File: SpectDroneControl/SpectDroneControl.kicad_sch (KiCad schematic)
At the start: 125 parts, among them J1 Conn_02x03_Counter_Clockwise, J1-1 Conn_01x04_Male, J1-2 Conn_01x04_Male, J3-1 Conn_01x01_Female, J3-2 Conn_01x01_Female, J3-3 Conn_01x01_Female, J3-4 Conn_01x01_Female, J3-5 Conn_01x01_Female, J3V1 Conn_01x01_Male, J5-1 Conn_01x01_Female, J5-2 Conn_01x01_Female, J5-3 Conn_01x01_Female, J5-4 Conn_01x01_Female, J5-5 Conn_01x01_Female, Q1 FDN340P, SW1 SW_SPDT, U1 Teensy4.1, U2 Teensy4.0, U3 NVT2010PW, U4 NVT2010PW, U5 NVT2010PW, U6 MCP112-450E/TO, U7 LM7805_SOT223

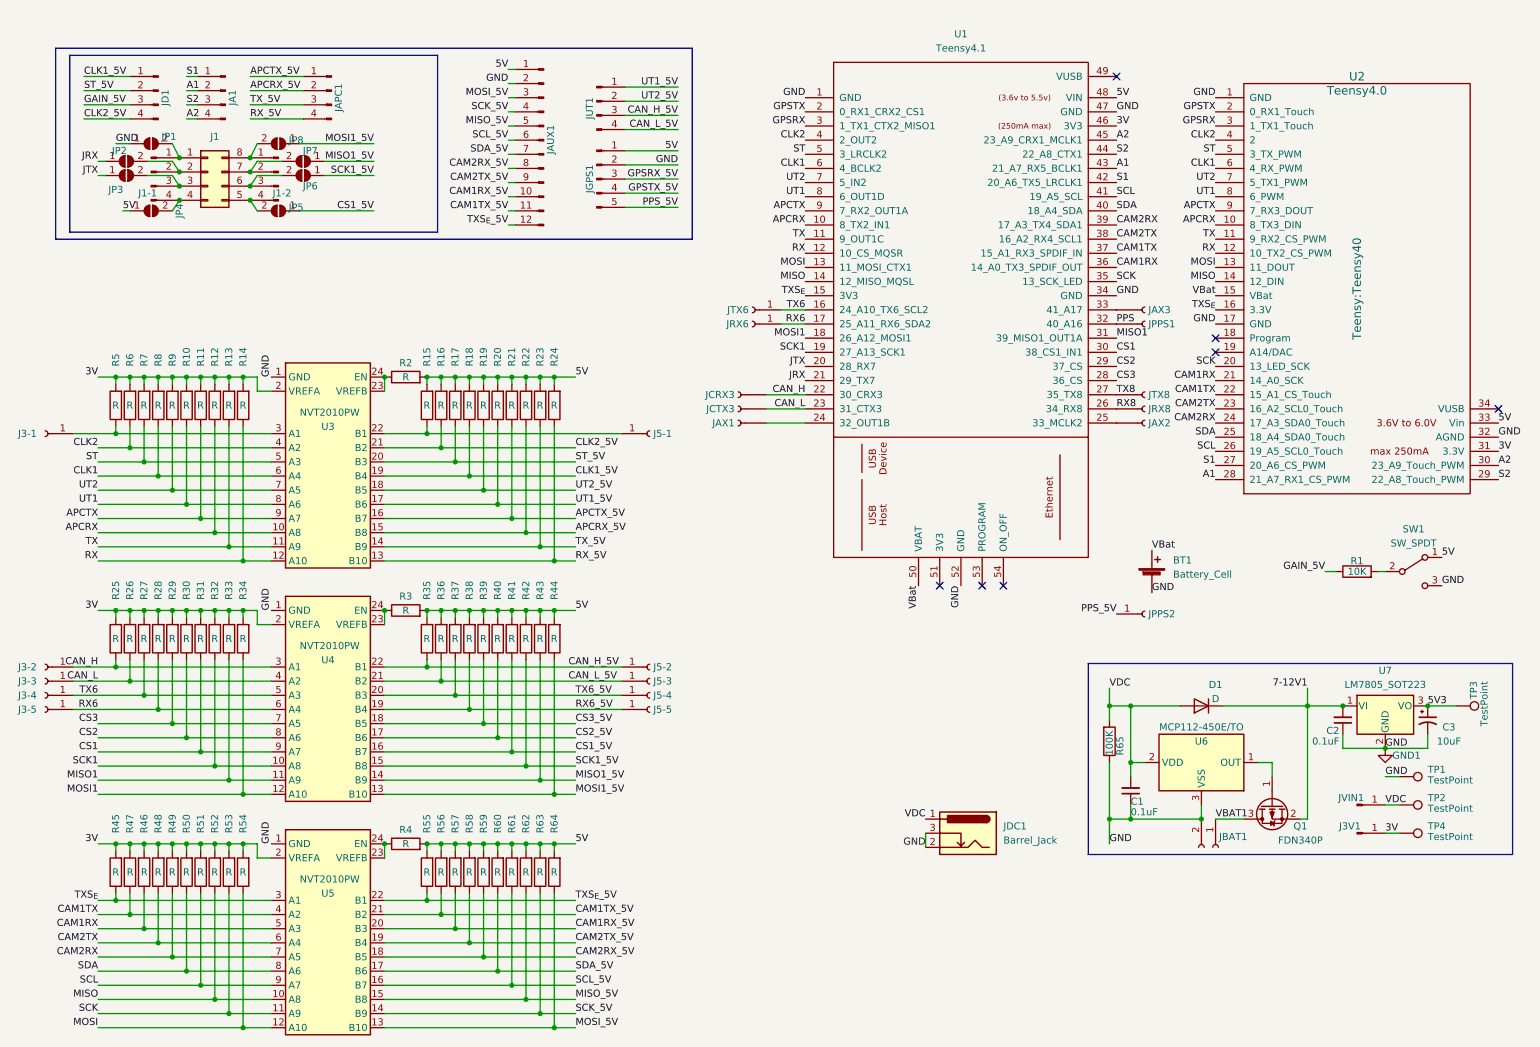
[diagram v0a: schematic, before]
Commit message: SpectDrone Development
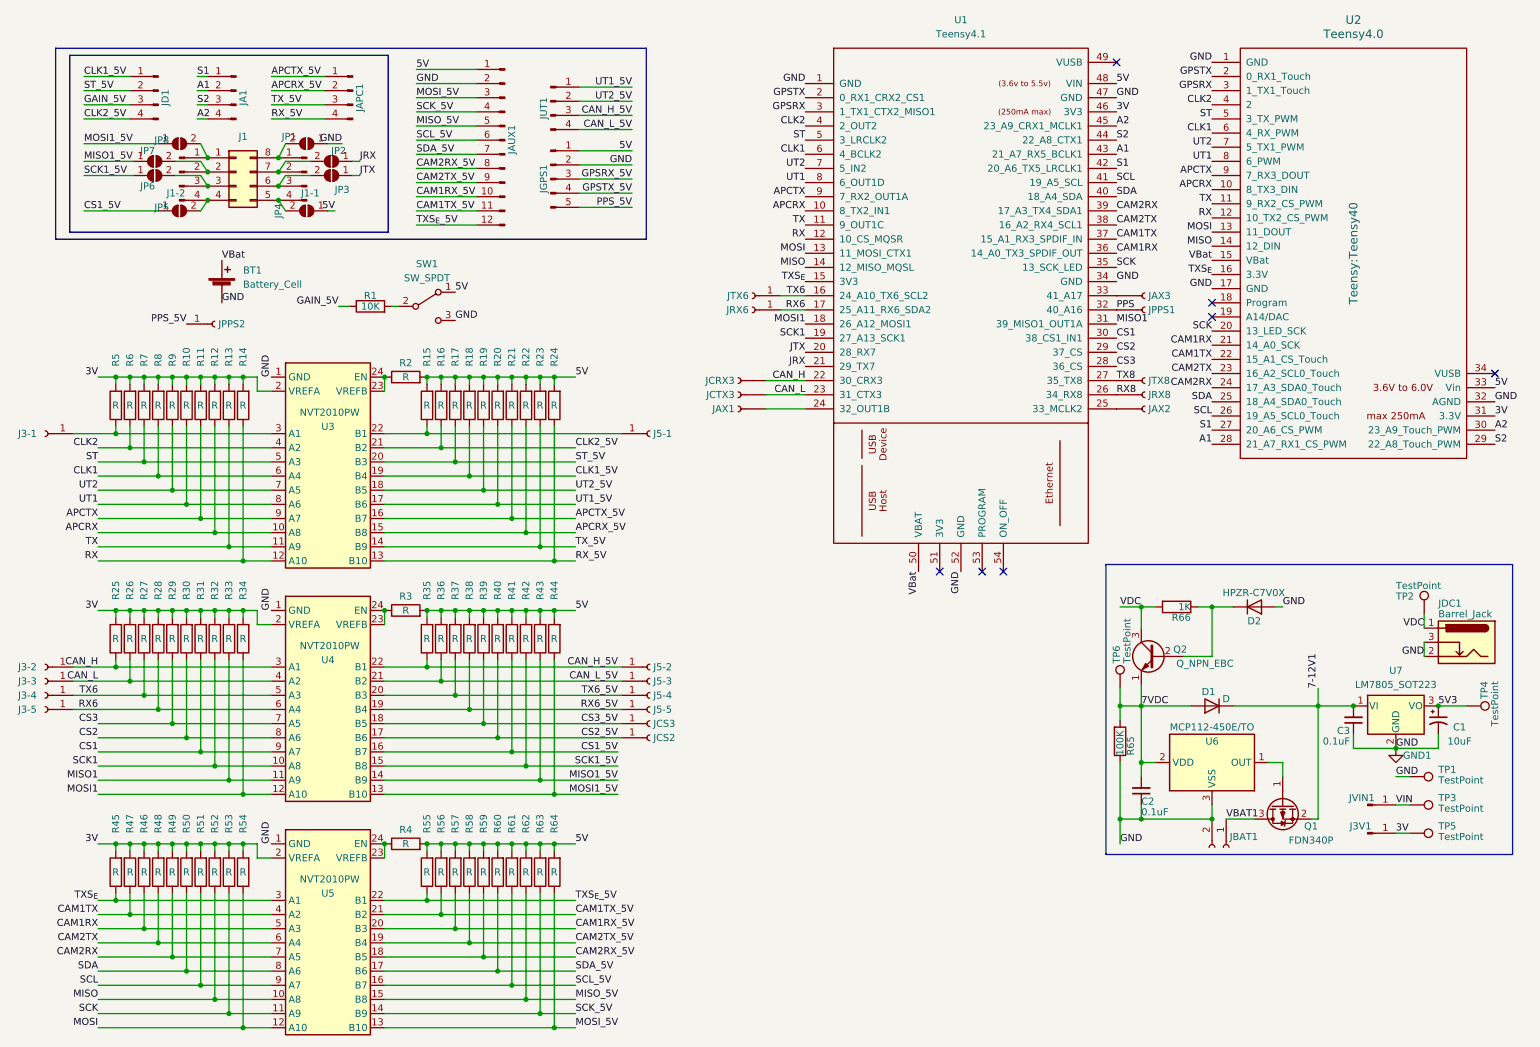
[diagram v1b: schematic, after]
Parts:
- added D2: HPZR-C7V0X, Diode_SMD:D_SOD-123F, symbol Device:D
- added JCS2, JCS3: Conn_01x01_Female, Connector_Wire:SolderWire-0.1sqmm_1x01_D0.4mm_OD1mm, symbol Connector:Conn_01x01_Female
- added Q2: Q_NPN_EBC, Package_TO_SOT_SMD:SOT-323_SC-70, symbol Device:Q_NPN_EBC
- added R66: 1K, Capacitor_SMD:C_0805_2012Metric, symbol Device:R
- added TP2, TP6: TestPoint, TestPoint:TestPoint_Keystone_5000-5004_Miniature, symbol Connector:TestPoint
- renumbered C3 to C1, C1 to C2, C2 to C3, TP2 to TP3, TP3 to TP4, TP4 to TP5
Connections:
- net CS2_5V: now also JCS2.1 (Pin_1)
- net CS3_5V: now also JCS3.1 (Pin_1)
- net GND1: now also D2.2 (A)
- net VDC: now also Q2.3 (C), R66.2, TP2.1; no longer C2.2, D1.2 (A), JVIN1.1 (Pin_1), R65.2, TP3.1, U6.2 (VDD)
- net at J1-1.3 (Pin_3), JP3.2 (B): now also J1.6 (Pin_6); no longer J1.3 (Pin_3)
- net at J1-1.1 (Pin_1), JP1.2 (B): now also J1.8 (Pin_8); no longer J1.1 (Pin_1)
- net at J1-1.2 (Pin_2), JP2.2 (B): now also J1.7 (Pin_7); no longer J1.2 (Pin_2)
- net at J1-1.4 (Pin_4), JP4.2 (B): now also J1.5 (Pin_5); no longer J1.4 (Pin_4)
- net at J1-2.4 (Pin_4), JP5.2 (B): now also J1.4 (Pin_4); no longer J1.5 (Pin_5)
- net at J1-2.3 (Pin_3), JP6.2 (B): now also J1.3 (Pin_3); no longer J1.6 (Pin_6)
- net at J1-2.2 (Pin_2), JP7.2 (B): now also J1.2 (Pin_2); no longer J1.7 (Pin_7)
- net at J1-2.1 (Pin_1), JP8.2 (B): now also J1.1 (Pin_1); no longer J1.8 (Pin_8)
- new net: D2.1 (K), Q2.2 (B), R66.1
- new net 7VDC: C2.2, D1.2 (A), Q2.1 (E), R65.2, TP6.1, U6.2 (VDD)
- new net VIN: JVIN1.1 (Pin_1), TP3.1
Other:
- moved on the sheet: BT1, C1, C2, C3, D1, J1, J1-1, J1-2, J3V1, JA1, JAPC1, JAUX1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

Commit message: SpectDrone Development
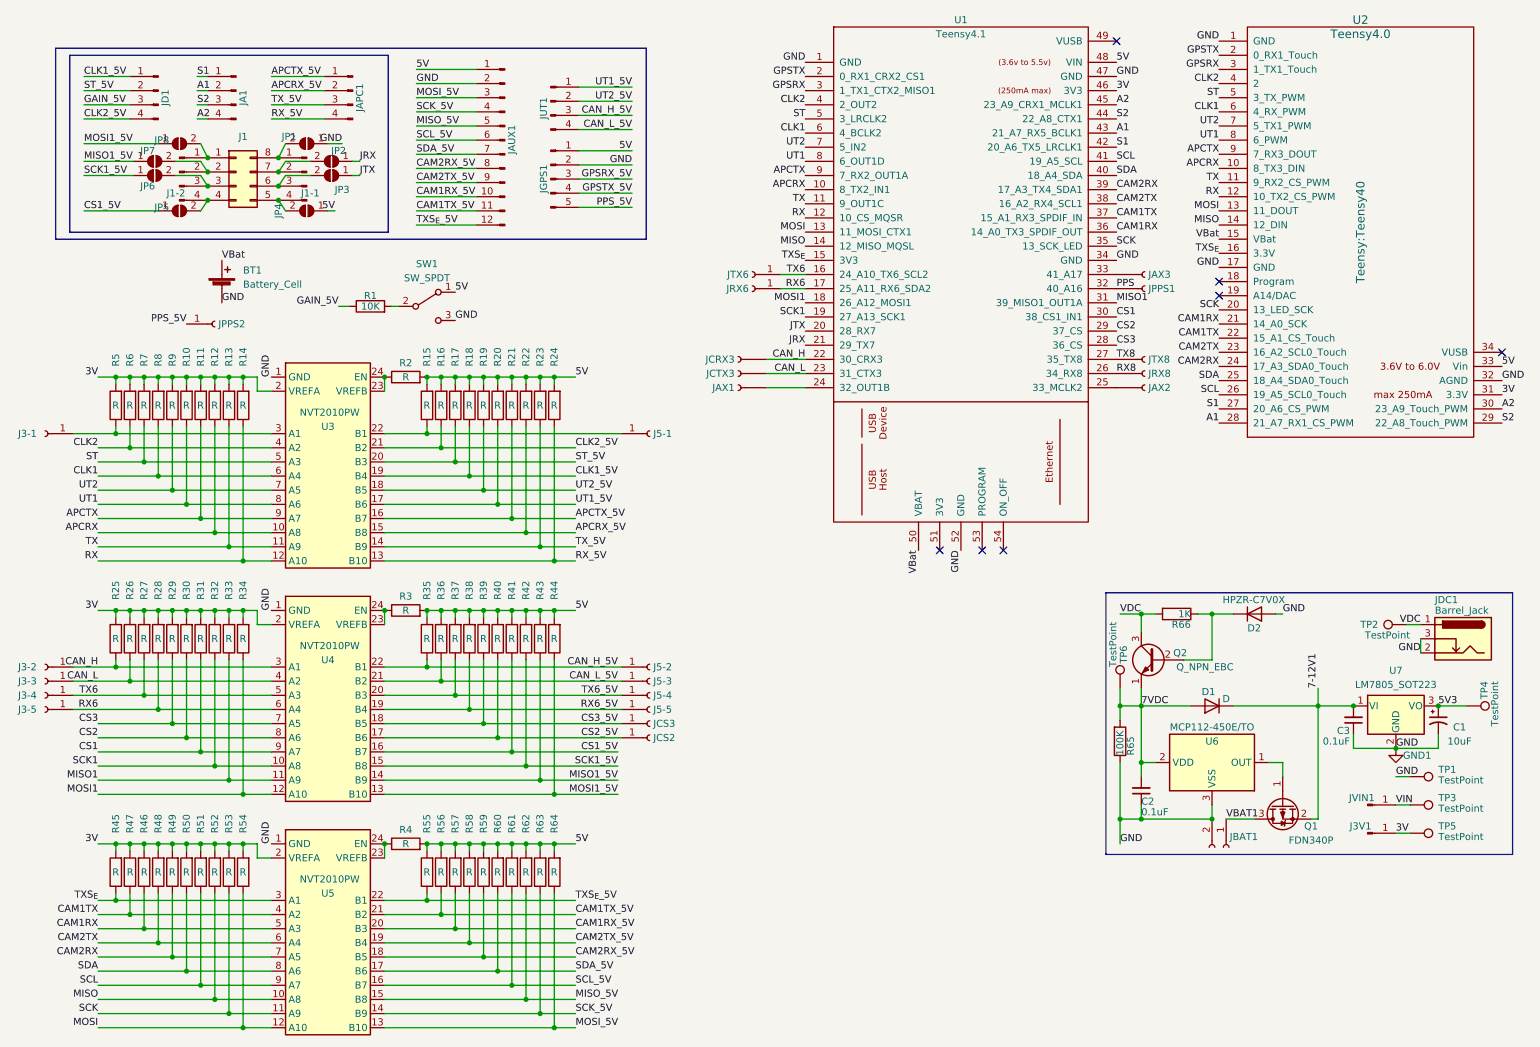
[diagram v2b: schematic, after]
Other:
- moved on the sheet: D2, JAX1, JAX2, JAX3, JCRX3, JCTX3, JDC1, JPPS1, JRX6, JRX8, JTX6, JTX8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
